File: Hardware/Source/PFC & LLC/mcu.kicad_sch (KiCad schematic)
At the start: 43 parts, among them J2 FLASH PROGRAM, J3 COMMAND LINE, SW1 RESET, U3 STM32F107RCT6, Y1 Crystal_25MHz_SMD-4PIN

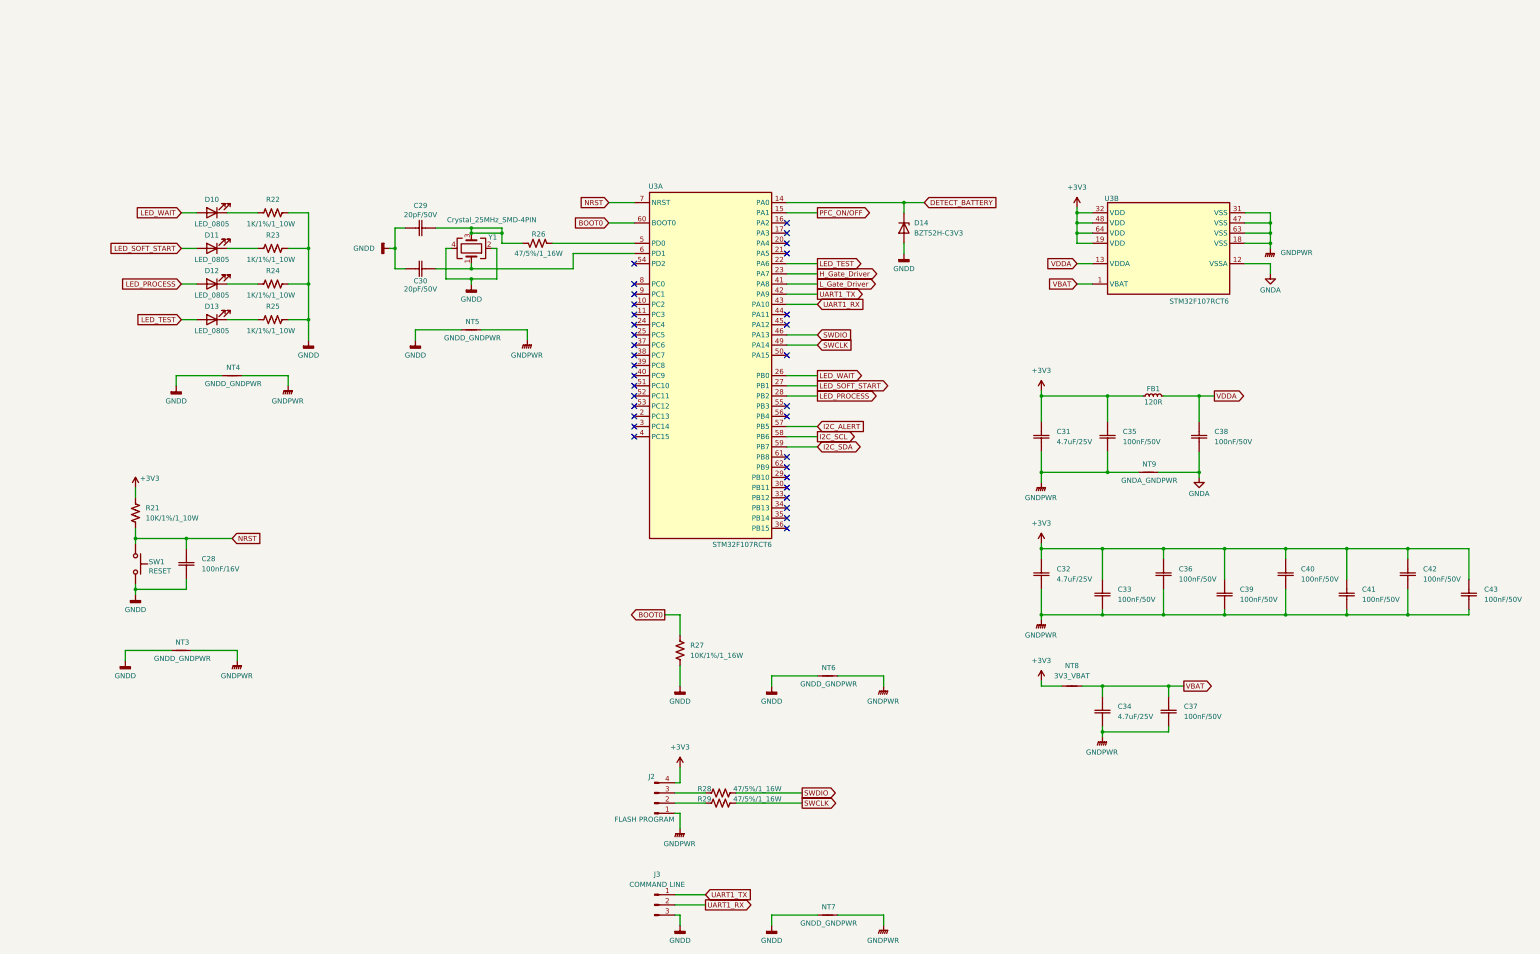
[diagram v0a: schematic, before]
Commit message: update lib, LLC
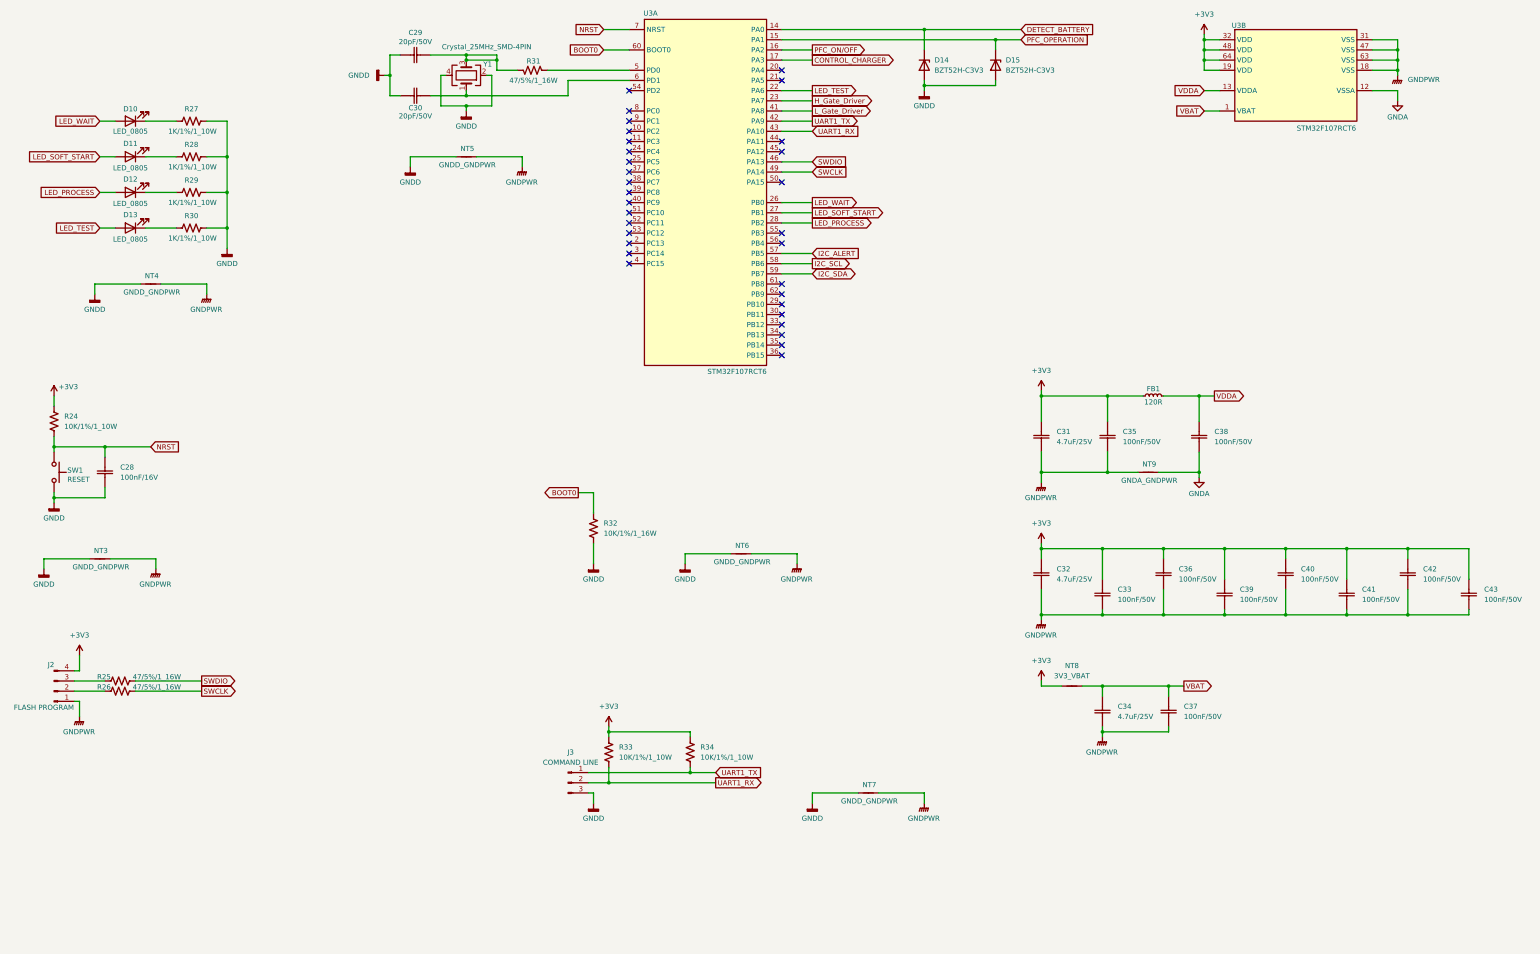
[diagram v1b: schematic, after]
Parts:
- removed R22, R23, R24, R25: 1K/1%/1_10W, charge_battery_footprint_lib:Res_0603, symbol charge_battery_sym_lib:Res_1K_0603_1%
- added D15: BZT52H-C3V3, charge_battery_footprint_lib:Diode_Zener_BZT52H, symbol charge_battery_sym_lib:BZT52H-C3V3
- added R27, R28, R29, R30: 1K/1%/1_10W, charge_battery_footprint_lib:Res_0603, symbol charge_battery_sym_lib:Res_1K_0603_1%
- added R33, R34: 10K/1%/1_10W, charge_battery_footprint_lib:Res_0603, symbol charge_battery_sym_lib:Res_10K_0603_1%
- renumbered R21 to R24, R28 to R25, R29 to R26, R26 to R31, R27 to R32
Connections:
- net +3V3: now also R33.2, R34.2
- net GNDD: now also D15.2 (A), R27.2, R28.2, R29.2, R30.2
- net PFC_ON/OFF: now also U3.16 (PA2); no longer U3.15 (PA1)
- net UART1_RX: now also R33.1
- net UART1_TX: now also R34.1
- net at D13.1 (K): now also R30.1
- net at D12.1 (K): now also R29.1
- net at D11.1 (K): now also R28.1
- net at D10.1 (K): now also R27.1
- net CONTROL_CHARGER: now reaches U3.17 (PA3)
- new net PFC_OPERATION: D15.1 (K), U3.15 (PA1)
- no-connect marks 34 -> 32
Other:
- moved on the sheet: C28, C29, C30, D11, D12, D13, D14, J2, J3, NT3, NT4, NT5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
